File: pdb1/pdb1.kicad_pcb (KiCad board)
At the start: 2 copper layers, 142.2 x 17.8 mm, 23 parts, among them P1 CONN_XT60, P2 CONN_XT60, P3 CONN_02X03, P4 CONN_02X03, P5 CONN_01X03, P6 CONN_XT60, P7 CONN_XT60, P8 CONN_XT60, Q2 BUK9Y4R8-60E, U1 INA169, U2 NSI45020AT1G, U3 NSI45020AT1G, U7 MIC5014, U8 NSI45020AT1G

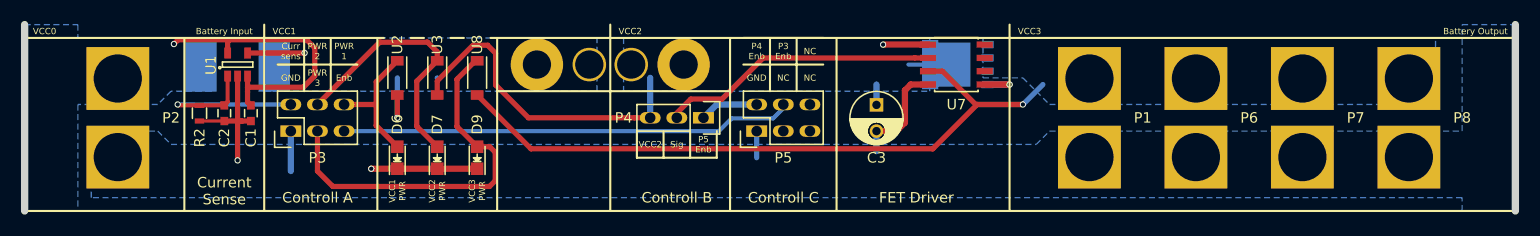
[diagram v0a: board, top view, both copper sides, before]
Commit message: test
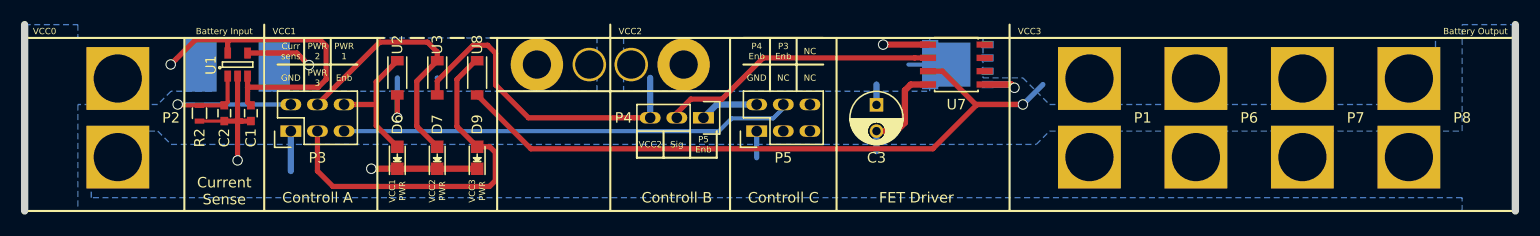
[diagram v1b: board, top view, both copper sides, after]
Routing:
- net /channel/in+: track 27.7 -> 31.3 mm
- net Net-(Q2-Pad4): track 4.48 -> 5.67 mm
- net /channel/fuse/in+: track 11.4 -> 12.3 mm
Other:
- net class Default: via_dia 0.6 -> 1; via_drill 0.4 -> 0.8
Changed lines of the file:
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@@
-(kicad_pcb (version 4) (host pcbnew 4.0.4-stable)
+(kicad_pcb (version 4) (host pcbnew 4.0.4+e1-6308~48~ubuntu16.04.1-stable)
   (general
     (links 51)
@@
     (thickness 1.6)
     (drawings 58)
-    (tracks 119)
+    (tracks 122)
     (zones 0)
     (modules 23)
@@
     (segment_width 0.2)
     (edge_width 0.7)
-    (via_size 0.6)
-    (via_drill 0.4)
+    (via_size 1)
+    (via_drill 0.8)
     (via_min_size 0.4)
     (via_min_drill 0.3)
@@
     (clearance 0.2)
     (trace_width 0.25)
-    (via_dia 0.6)
-    (via_drill 0.4)
+    (via_dia 1)
+    (via_drill 0.8)
     (uvia_dia 0.3)
     (uvia_drill 0.1)
@@
   (gr_line (start 205.74 50.8) (end 205.74 68.58) (layer Edge.Cuts) (width 0.7))
   (segment (start 102.861339 55.888661) (end 102.867466 55.894788) (width 0.5) (layer B.Cu) (net 0))
-  (segment (start 84.77 56.769) (end 90.09998 56.769) (width 0.5) (layer F.Cu) (net 1))
-  (segment (start 90.398599 52.248087) (end 82.8675 52.248087) (width 0.5) (layer F.Cu) (net 1))
-  (segment (start 91.184452 53.03394) (end 90.398599 52.248087) (width 0.5) (layer F.Cu) (net 1))
-  (segment (start 91.184452 55.684528) (end 91.184452 53.03394) (width 0.5) (layer F.Cu) (net 1))
-  (segment (start 90.09998 56.769) (end 91.184452 55.684528) (width 0.5) (layer F.Cu) (net 1))
+  (segment (start 84.77 56.769) (end 91.520335 56.769) (width 0.5) (layer F.Cu) (net 1))
+  (segment (start 91.520335 56.769) (end 92.267073 56.022262) (width 0.5) (layer F.Cu) (net 1))
+  (segment (start 92.267073 52.831438) (end 91.683722 52.248087) (width 0.5) (layer F.Cu) (net 1))
+  (segment (start 92.267073 56.022262) (end 92.267073 52.831438) (width 0.5) (layer F.Cu) (net 1))
+  (segment (start 91.683722 52.248087) (end 82.8675 52.248087) (width 0.5) (layer F.Cu) (net 1))
+  (segment (start 77.939278 54.101997) (end 77.439279 54.601996) (width 0.5) (layer F.Cu) (net 1))
+  (segment (start 79.793188 52.248087) (end 77.939278 54.101997) (width 0.5) (layer F.Cu) (net 1))
+  (segment (start 82.8675 52.248087) (end 79.793188 52.248087) (width 0.5) (layer F.Cu) (net 1))
+  (via (at 77.439279 54.601996) (size 1) (drill 0.8) (layers F.Cu B.Cu) (net 1))
   (segment (start 84.77 56.769) (end 84.77 57.2135) (width 0.5) (layer F.Cu) (net 1))
   (segment (start 84.77 55.71) (end 84.77 56.769) (width 0.5) (layer F.Cu) (net 1))
-  (segment (start 78.044102 52.350562) (end 77.744103 52.650561) (width 0.5) (layer F.Cu) (net 1))
-  (segment (start 78.146577 52.248087) (end 78.044102 52.350562) (width 0.5) (layer F.Cu) (net 1))
-  (segment (start 82.8675 52.248087) (end 78.146577 52.248087) (width 0.5) (layer F.Cu) (net 1))
-  (via (at 77.744103 52.650561) (size 0.6) (drill 0.4) (layers F.Cu B.Cu) (net 1))
   (segment (start 82.87 53.51) (end 82.87 52.48) (width 0.5) (layer F.Cu) (net 1))
   (segment (start 82.8675 52.4775) (end 82.8675 52.248087) (width 0.5) (layer F.Cu) (net 1))
@@
   (segment (start 84.215 60.001086) (end 84.208586 60.0075) (width 0.5) (layer F.Cu) (net 2))
   (segment (start 84.208586 60.0075) (end 83.82 60.0075) (width 0.5) (layer F.Cu) (net 2))
-  (via (at 83.82 63.754) (size 0.6) (drill 0.4) (layers F.Cu B.Cu) (net 2))
+  (via (at 83.82 63.754) (size 1) (drill 0.8) (layers F.Cu B.Cu) (net 2))
   (segment (start 96.575773 64.54902) (end 96.574716 64.547963) (width 0.6) (layer F.Cu) (net 2))
   (segment (start 99.06 64.54902) (end 96.575773 64.54902) (width 0.6) (layer F.Cu) (net 2))
-  (via (at 96.574716 64.547963) (size 0.6) (drill 0.4) (layers F.Cu B.Cu) (net 2))
+  (via (at 96.574716 64.547963) (size 1) (drill 0.8) (layers F.Cu B.Cu) (net 2))
   (segment (start 102.87 64.54902) (end 99.06 64.54902) (width 0.6) (layer F.Cu) (net 2))
   (segment (start 106.68 64.54902) (end 102.87 64.54902) (width 0.6) (layer F.Cu) (net 2))
@@
   (segment (start 78.105 58.42) (end 88.330002 58.42) (width 0.4) (layer B.Cu) (net 3))
   (segment (start 88.330002 58.42) (end 88.9 58.42) (width 0.4) (layer B.Cu) (net 3))
-  (via (at 78.105 58.42) (size 0.6) (drill 0.4) (layers F.Cu B.Cu) (net 3))
+  (via (at 78.105 58.42) (size 1) (drill 0.8) (layers F.Cu B.Cu) (net 3))
   (segment (start 102.87 57.515) (end 102.87 56.179998) (width 0.5) (layer F.Cu) (net 4))
   (segment (start 102.87 56.179998) (end 106.284563 52.765435) (width 0.5) (layer F.Cu) (net 4))
@@
   (segment (start 152.1 54.61) (end 149.9 54.61) (width 0.4) (layer B.Cu) (net 4))
   (segment (start 149.7 52.705) (end 145.415 52.705) (width 0.6) (layer F.Cu) (net 4))
-  (via (at 145.415 52.705) (size 0.6) (drill 0.4) (layers F.Cu B.Cu) (net 4))
+  (via (at 145.415 52.705) (size 1) (drill 0.8) (layers F.Cu B.Cu) (net 4))
   (segment (start 97.044609 60.435589) (end 97.044609 58.42) (width 0.5) (layer F.Cu) (net 5))
   (segment (start 97.044609 58.42) (end 97.044609 56.260391) (width 0.5) (layer F.Cu) (net 5))
@@
   (segment (start 92.911879 66.241879) (end 91.44 64.77) (width 0.5) (layer F.Cu) (net 7))
   (segment (start 91.44 64.77) (end 91.44 60.96) (width 0.5) (layer F.Cu) (net 7))
+  (segment (start 90.131328 54.160988) (end 90.631327 54.660987) (width 0.5) (layer F.Cu) (net 8))
+  (segment (start 89.48034 53.51) (end 90.131328 54.160988) (width 0.5) (layer F.Cu) (net 8))
+  (segment (start 84.77 53.51) (end 89.48034 53.51) (width 0.5) (layer F.Cu) (net 8))
+  (via (at 90.631327 54.660987) (size 1) (drill 0.8) (layers F.Cu B.Cu) (net 8))
   (segment (start 99.06 59.69) (end 99.06 55.88) (width 0.5) (layer B.Cu) (net 8))
   (segment (start 99.06 57.515) (end 99.06 59.69) (width 0.5) (layer F.Cu) (net 8))
-  (via (at 99.06 59.69) (size 0.6) (drill 0.4) (layers F.Cu B.Cu) (net 8))
-  (segment (start 90.198965 53.51) (end 90.211015 53.49795) (width 0.5) (layer F.Cu) (net 8))
-  (segment (start 84.77 53.51) (end 90.198965 53.51) (width 0.5) (layer F.Cu) (net 8))
-  (via (at 90.211015 53.49795) (size 0.6) (drill 0.4) (layers F.Cu B.Cu) (net 8))
-  (segment (start 158.75 58.42) (end 154.381826 58.42) (width 0.5) (layer F.Cu) (net 9))
+  (via (at 99.06 59.69) (size 1) (drill 0.8) (layers F.Cu B.Cu) (net 8))
+  (segment (start 158.75 58.42) (end 160.655 56.515) (width 0.5) (layer B.Cu) (net 9))
+  (segment (start 154.25 58.42) (end 151.075 55.245) (width 0.5) (layer F.Cu) (net 9))
+  (segment (start 158.75 58.42) (end 154.25 58.42) (width 0.5) (layer F.Cu) (net 9))
+  (segment (start 151.075 55.245) (end 149.7 55.245) (width 0.5) (layer F.Cu) (net 9))
+  (segment (start 111.814097 62.649097) (end 106.68 57.515) (width 0.5) (layer F.Cu) (net 9))
   (segment (start 150.152729 62.649097) (end 111.814097 62.649097) (width 0.5) (layer F.Cu) (net 9))
   (segment (start 154.381826 58.42) (end 150.152729 62.649097) (width 0.5) (layer F.Cu) (net 9))
-  (segment (start 111.814097 62.649097) (end 106.68 57.515) (width 0.5) (layer F.Cu) (net 9))
-  (segment (start 158.75 58.42) (end 154.25 58.42) (width 0.5) (layer F.Cu) (net 9))
-  (segment (start 154.25 58.42) (end 151.075 55.245) (width 0.5) (layer F.Cu) (net 9))
-  (segment (start 151.075 55.245) (end 149.7 55.245) (width 0.5) (layer F.Cu) (net 9))
-  (segment (start 158.75 58.42) (end 160.655 56.515) (width 0.5) (layer B.Cu) (net 9))
-  (via (at 158.75 58.42) (size 0.6) (drill 0.4) (layers F.Cu B.Cu) (net 9))
-  (segment (start 157.48 56.515) (end 155.375 56.515) (width 0.6) (layer B.Cu) (net 10))
-  (segment (start 155.1 56.515) (end 157.48 56.515) (width 0.6) (layer F.Cu) (net 10))
-  (via (at 157.48 56.515) (size 0.6) (drill 0.4) (layers F.Cu B.Cu) (net 10))
+  (segment (start 158.75 58.42) (end 154.381826 58.42) (width 0.5) (layer F.Cu) (net 9))
+  (via (at 158.75 58.42) (size 1) (drill 0.8) (layers F.Cu B.Cu) (net 9))
+  (segment (start 157.635538 56.515) (end 157.945139 56.824601) (width 0.6) (layer F.Cu) (net 10))
+  (segment (start 155.1 56.515) (end 157.635538 56.515) (width 0.6) (layer F.Cu) (net 10))
+  (segment (start 157.635538 56.515) (end 157.945139 56.824601) (width 0.6) (layer B.Cu) (net 10))
+  (segment (start 155.375 56.515) (end 157.635538 56.515) (width 0.6) (layer B.Cu) (net 10))
+  (via (at 157.945139 56.824601) (size 1) (drill 0.8) (layers F.Cu B.Cu) (net 10))
   (segment (start 93.98 60.96) (end 129.746733 60.96) (width 0.4) (layer B.Cu) (net 11))
   (segment (start 129.746733 60.96) (end 130.964502 59.742231) (width 0.4) (layer B.Cu) (net 11))
